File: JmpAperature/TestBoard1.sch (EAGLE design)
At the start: 4 parts

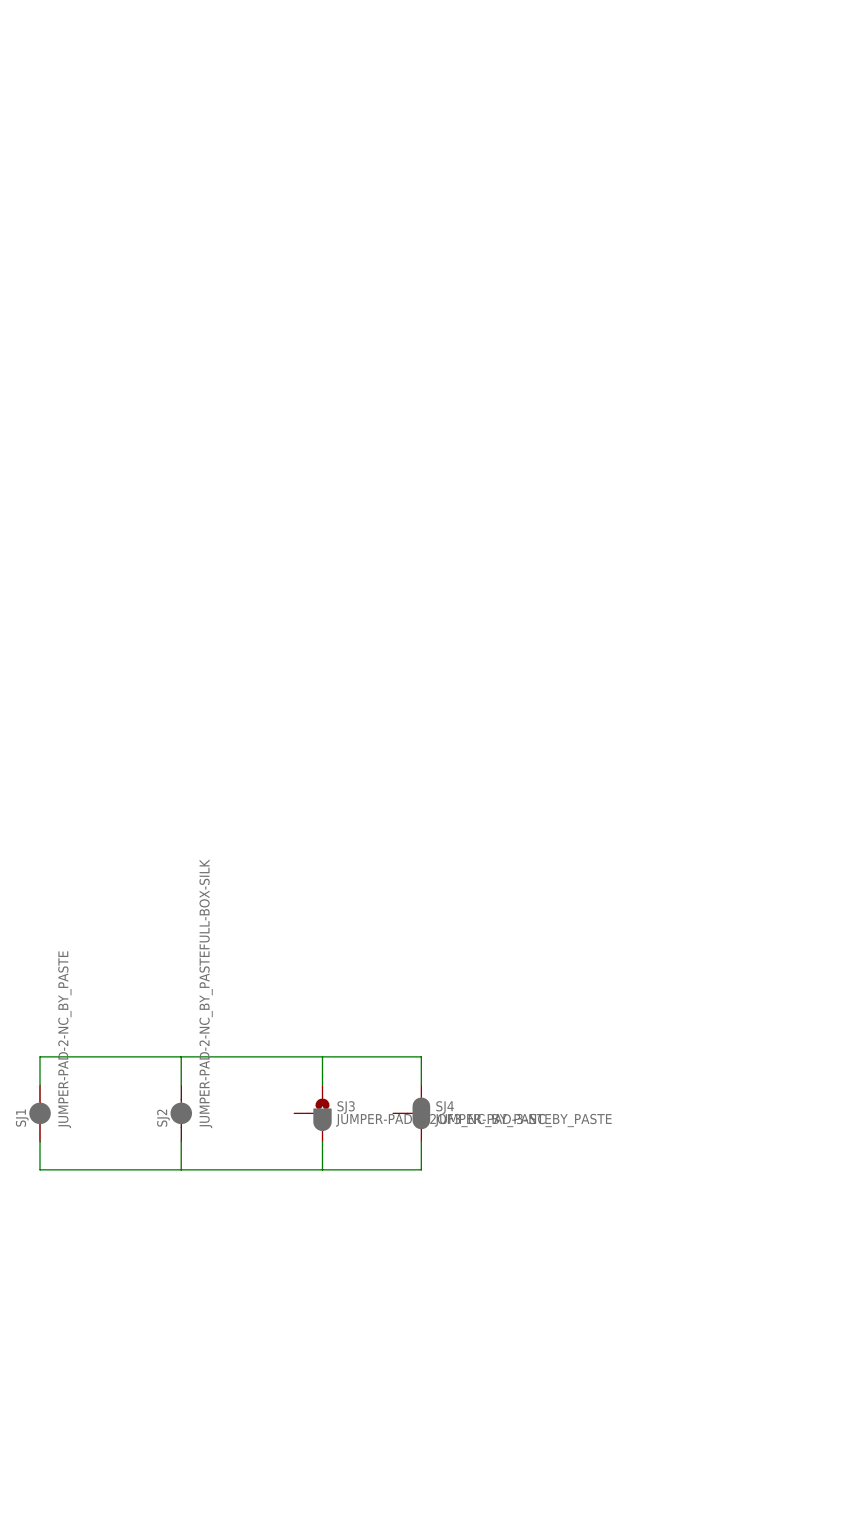
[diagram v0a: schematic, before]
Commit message: updated
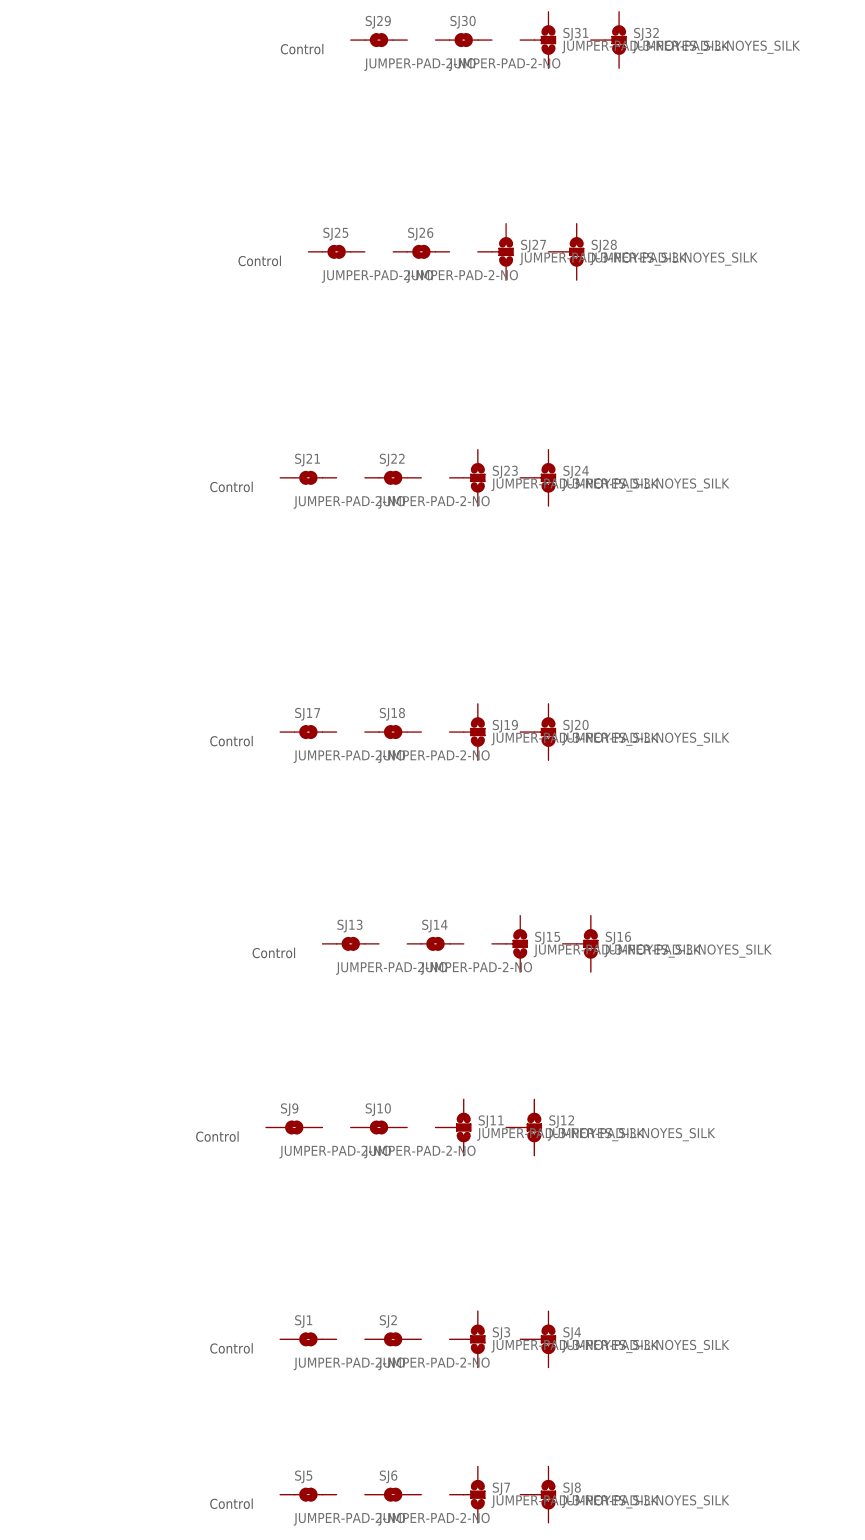
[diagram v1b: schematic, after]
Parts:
- added SJ10, SJ13, SJ14, SJ17, SJ18, SJ21, SJ22, SJ25, SJ26, SJ29, SJ30, SJ5, SJ6, SJ9: JUMPER-PAD-2-NO, TestAperatures:JUMPER-PAD-2-NO
- added SJ11, SJ12, SJ15, SJ16, SJ19, SJ20, SJ23, SJ24, SJ27, SJ28, SJ31, SJ32, SJ7, SJ8: JUMPER-PAD-3-NOYES_SILK, TestAperatures:JUMPER-PAD-3-NOYES_SILK
- SJ1: value JUMPER-PAD-2-NC_BY_PASTE -> JUMPER-PAD-2-NO; device TestAperatures:JUMPER-PAD-2-NC_BY_PASTE -> TestAperatures:JUMPER-PAD-2-NO
- SJ2: value JUMPER-PAD-2-NC_BY_PASTEFULL-BOX-SILK -> JUMPER-PAD-2-NO; device TestAperatures:JUMPER-PAD-2-NC_BY_PASTEFULL-BOX-SILK -> TestAperatures:JUMPER-PAD-2-NO
- SJ3: value JUMPER-PAD-3-2OF3_NC_BY_PASTE -> JUMPER-PAD-3-NOYES_SILK; device TestAperatures:JUMPER-PAD-3-2OF3_NC_BY_PASTE -> TestAperatures:JUMPER-PAD-3-NOYES_SILK
- SJ4: value JUMPER-PAD-3-NC_BY_PASTE -> JUMPER-PAD-3-NOYES_SILK; device TestAperatures:JUMPER-PAD-3-NC_BY_PASTE -> TestAperatures:JUMPER-PAD-3-NOYES_SILK
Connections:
- removed net GND: SJ1.1, SJ2.1, SJ3.3, SJ4.3
- removed net PWR: SJ1.2, SJ2.2, SJ3.1, SJ4.1
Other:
- note added: "Control"
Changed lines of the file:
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@@
 </classes>
 <parts>
-<part name="SJ1" library="TestAperatures" deviceset="JUMPER-PAD-2-NC_BY_PASTE" device=""/>
-<part name="SJ2" library="TestAperatures" deviceset="JUMPER-PAD-2-NC_BY_PASTE" device="FULL-BOX-SILK"/>
-<part name="SJ3" library="TestAperatures" deviceset="JUMPER-PAD-3-2OF3_NC_BY_PASTE" device=""/>
-<part name="SJ4" library="TestAperatures" deviceset="JUMPER-PAD-3-NC_BY_PASTE" device=""/>
+<part name="SJ5" library="TestAperatures" deviceset="JUMPER-PAD-2-NO" device=""/>
+<part name="SJ6" library="TestAperatures" deviceset="JUMPER-PAD-2-NO" device=""/>
+<part name="SJ7" library="TestAperatures" deviceset="JUMPER-PAD-3-NO" device="YES_SILK"/>
+<part name="SJ8" library="TestAperatures" deviceset="JUMPER-PAD-3-NO" device="YES_SILK"/>
+<part name="SJ1" library="TestAperatures" deviceset="JUMPER-PAD-2-NO" device=""/>
+<part name="SJ2" library="TestAperatures" deviceset="JUMPER-PAD-2-NO" device=""/>
+<part name="SJ3" library="TestAperatures" deviceset="JUMPER-PAD-3-NO" device="YES_SILK"/>
+<part name="SJ4" library="TestAperatures" deviceset="JUMPER-PAD-3-NO" device="YES_SILK"/>
+<part name="SJ9" library="TestAperatures" deviceset="JUMPER-PAD-2-NO" device=""/>
+<part name="SJ10" library="TestAperatures" deviceset="JUMPER-PAD-2-NO" device=""/>
+<part name="SJ11" library="TestAperatures" deviceset="JUMPER-PAD-3-NO" device="YES_SILK"/>
+<part name="SJ12" library="TestAperatures" deviceset="JUMPER-PAD-3-NO" device="YES_SILK"/>
+<part name="SJ13" library="TestAperatures" deviceset="JUMPER-PAD-2-NO" device=""/>
+<part name="SJ14" library="TestAperatures" deviceset="JUMPER-PAD-2-NO" device=""/>
+<part name="SJ15" library="TestAperatures" deviceset="JUMPER-PAD-3-NO" device="YES_SILK"/>
+<part name="SJ16" library="TestAperatures" deviceset="JUMPER-PAD-3-NO" device="YES_SILK"/>
+<part name="SJ17" library="TestAperatures" deviceset="JUMPER-PAD-2-NO" device=""/>
+<part name="SJ18" library="TestAperatures" deviceset="JUMPER-PAD-2-NO" device=""/>
+<part name="SJ19" library="TestAperatures" deviceset="JUMPER-PAD-3-NO" device="YES_SILK"/>
+<part name="SJ20" library="TestAperatures" deviceset="JUMPER-PAD-3-NO" device="YES_SILK"/>
+<part name="SJ21" library="TestAperatures" deviceset="JUMPER-PAD-2-NO" device=""/>
+<part name="SJ22" library="TestAperatures" deviceset="JUMPER-PAD-2-NO" device=""/>
+<part name="SJ23" library="TestAperatures" deviceset="JUMPER-PAD-3-NO" device="YES_SILK"/>
+<part name="SJ24" library="TestAperatures" deviceset="JUMPER-PAD-3-NO" device="YES_SILK"/>
+<part name="SJ25" library="TestAperatures" deviceset="JUMPER-PAD-2-NO" device=""/>
+<part name="SJ26" library="TestAperatures" deviceset="JUMPER-PAD-2-NO" device=""/>
+<part name="SJ27" library="TestAperatures" deviceset="JUMPER-PAD-3-NO" device="YES_SILK"/>
+<part name="SJ28" library="TestAperatures" deviceset="JUMPER-PAD-3-NO" device="YES_SILK"/>
+<part name="SJ29" library="TestAperatures" deviceset="JUMPER-PAD-2-NO" device=""/>
+<part name="SJ30" library="TestAperatures" deviceset="JUMPER-PAD-2-NO" device=""/>
+<part name="SJ31" library="TestAperatures" deviceset="JUMPER-PAD-3-NO" device="YES_SILK"/>
+<part name="SJ32" library="TestAperatures" deviceset="JUMPER-PAD-3-NO" device="YES_SILK"/>
 </parts>
 <sheets>
 <sheet>
 <plain>
+<text x="15.24" y="15.24" size="1.778" layer="97">Control</text>
+<text x="15.24" y="43.18" size="1.778" layer="97">Control</text>
+<text x="12.7" y="81.28" size="1.778" layer="97">Control</text>
+<text x="22.86" y="114.3" size="1.778" layer="97">Control</text>
+<text x="15.24" y="152.4" size="1.778" layer="97">Control</text>
+<text x="15.24" y="198.12" size="1.778" layer="97">Control</text>
+<text x="20.32" y="238.76" size="1.778" layer="97">Control</text>
+<text x="27.94" y="276.86" size="1.778" layer="97">Control</text>
 </plain>
 <instances>
-<instance part="SJ1" gate="G$1" x="-15.24" y="86.36" rot="R90"/>
-<instance part="SJ2" gate="G$1" x="10.16" y="86.36" rot="R90"/>
-<instance part="SJ3" gate="G$1" x="35.56" y="86.36"/>
-<instance part="SJ4" gate="G$1" x="53.34" y="86.36"/>
+<instance part="SJ5" gate="G$1" x="33.02" y="17.78"/>
+<instance part="SJ6" gate="G$1" x="48.26" y="17.78"/>
+<instance part="SJ7" gate="G$1" x="63.5" y="17.78"/>
+<instance part="SJ8" gate="G$1" x="76.2" y="17.78"/>
+<instance part="SJ1" gate="G$1" x="33.02" y="45.72"/>
+<instance part="SJ2" gate="G$1" x="48.26" y="45.72"/>
+<instance part="SJ3" gate="G$1" x="63.5" y="45.72"/>
+<instance part="SJ4" gate="G$1" x="76.2" y="45.72"/>
+<instance part="SJ9" gate="G$1" x="30.48" y="83.82"/>
+<instance part="SJ10" gate="G$1" x="45.72" y="83.82"/>
+<instance part="SJ11" gate="G$1" x="60.96" y="83.82"/>
+<instance part="SJ12" gate="G$1" x="73.66" y="83.82"/>
+<instance part="SJ13" gate="G$1" x="40.64" y="116.84"/>
+<instance part="SJ14" gate="G$1" x="55.88" y="116.84"/>
+<instance part="SJ15" gate="G$1" x="71.12" y="116.84"/>
+<instance part="SJ16" gate="G$1" x="83.82" y="116.84"/>
+<instance part="SJ17" gate="G$1" x="33.02" y="154.94"/>
+<instance part="SJ18" gate="G$1" x="48.26" y="154.94"/>
+<instance part="SJ19" gate="G$1" x="63.5" y="154.94"/>
+<instance part="SJ20" gate="G$1" x="76.2" y="154.94"/>
+<instance part="SJ21" gate="G$1" x="33.02" y="200.66"/>
+<instance part="SJ22" gate="G$1" x="48.26" y="200.66"/>
+<instance part="SJ23" gate="G$1" x="63.5" y="200.66"/>
+<instance part="SJ24" gate="G$1" x="76.2" y="200.66"/>
+<instance part="SJ25" gate="G$1" x="38.1" y="241.3"/>
+<instance part="SJ26" gate="G$1" x="53.34" y="241.3"/>
+<instance part="SJ27" gate="G$1" x="68.58" y="241.3"/>
+<instance part="SJ28" gate="G$1" x="81.28" y="241.3"/>
+<instance part="SJ29" gate="G$1" x="45.72" y="279.4"/>
+<instance part="SJ30" gate="G$1" x="60.96" y="279.4"/>
+<instance part="SJ31" gate="G$1" x="76.2" y="279.4"/>
+<instance part="SJ32" gate="G$1" x="88.9" y="279.4"/>
 </instances>
 <busses>
 </busses>
 <nets>
-<net name="PWR" class="0">
-<segment>
-<pinref part="SJ1" gate="G$1" pin="2"/>
-<wire x1="-15.24" y1="91.44" x2="-15.24" y2="96.52" width="0.1524" layer="91"/>
-<wire x1="-15.24" y1="96.52" x2="10.16" y2="96.52" width="0.1524" layer="91"/>
-<pinref part="SJ2" gate="G$1" pin="2"/>
-<wire x1="10.16" y1="91.44" x2="10.16" y2="96.52" width="0.1524" layer="91"/>
-<pinref part="SJ4" gate="G$1" pin="1"/>
-<wire x1="10.16" y1="96.52" x2="35.56" y2="96.52" width="0.1524" layer="91"/>
-<wire x1="35.56" y1="96.52" x2="53.34" y2="96.52" width="0.1524" layer="91"/>
-<wire x1="53.34" y1="96.52" x2="53.34" y2="91.44" width="0.1524" layer="91"/>
-<pinref part="SJ3" gate="G$1" pin="1"/>
-<wire x1="35.56" y1="96.52" x2="35.56" y2="91.44" width="0.1524" layer="91"/>
-</segment>
-</net>
-<net name="GND" class="0">
-<segment>
-<pinref part="SJ4" gate="G$1" pin="3"/>
-<wire x1="53.34" y1="81.28" x2="53.34" y2="76.2" width="0.1524" layer="91"/>
-<wire x1="53.34" y1="76.2" x2="35.56" y2="76.2" width="0.1524" layer="91"/>
-<pinref part="SJ1" gate="G$1" pin="1"/>
-<wire x1="35.56" y1="76.2" x2="10.16" y2="76.2" width="0.1524" layer="91"/>
-<wire x1="-15.24" y1="81.28" x2="-15.24" y2="76.2" width="0.1524" layer="91"/>
-<wire x1="-15.24" y1="76.2" x2="10.16" y2="76.2" width="0.1524" layer="91"/>
-<pinref part="SJ2" gate="G$1" pin="1"/>
-<wire x1="10.16" y1="76.2" x2="10.16" y2="81.28" width="0.1524" layer="91"/>
-<pinref part="SJ3" gate="G$1" pin="3"/>
-<wire x1="35.56" y1="81.28" x2="35.56" y2="76.2" width="0.1524" layer="91"/>
-</segment>
-</net>
 </nets>
 </sheet>

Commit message: First row plus footprints
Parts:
- added SJ100, SJ103, SJ104, SJ107, SJ108, SJ111, SJ112, SJ115, SJ116, SJ119, SJ120, SJ123, SJ124, SJ127, SJ128, SJ155, SJ156, SJ159, SJ160, SJ163, SJ164, SJ35, SJ36, SJ39, SJ40, SJ43, SJ44, SJ47, SJ48, SJ51, SJ52, SJ55, SJ56, SJ59, SJ60, SJ63, SJ64, SJ67, SJ68, SJ71, SJ72, SJ75, SJ76, SJ79, SJ80, SJ83, SJ84, SJ87, SJ88, SJ91, SJ92, SJ95, SJ96, SJ99: JUMPER-PAD-3-NOYES_SILK, TestAperatures:JUMPER-PAD-3-NOYES_SILK
- added SJ101, SJ102, SJ105, SJ106, SJ109, SJ110, SJ113, SJ114, SJ117, SJ118, SJ121, SJ122, SJ125, SJ126, SJ153, SJ154, SJ157, SJ158, SJ161, SJ162, SJ33, SJ34, SJ37, SJ38, SJ41, SJ42, SJ45, SJ46, SJ49, SJ50, SJ53, SJ54, SJ57, SJ58, SJ61, SJ62, SJ65, SJ66, SJ69, SJ70, SJ73, SJ74, SJ77, SJ78, SJ81, SJ82, SJ85, SJ86, SJ89, SJ90, SJ93, SJ94, SJ97, SJ98: JUMPER-PAD-2-NO, TestAperatures:JUMPER-PAD-2-NO
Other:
- moved on the sheet: SJ1, SJ10, SJ11, SJ12, SJ13, SJ14, SJ15, SJ16, SJ17, SJ18, SJ19, SJ2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
